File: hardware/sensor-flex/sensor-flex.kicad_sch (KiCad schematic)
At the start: 34 parts, among them IC1 VCNL4040M3OE, IC2 VCNL4040M3OE, J1 Conn_01x05, U1 PCA9546APWR

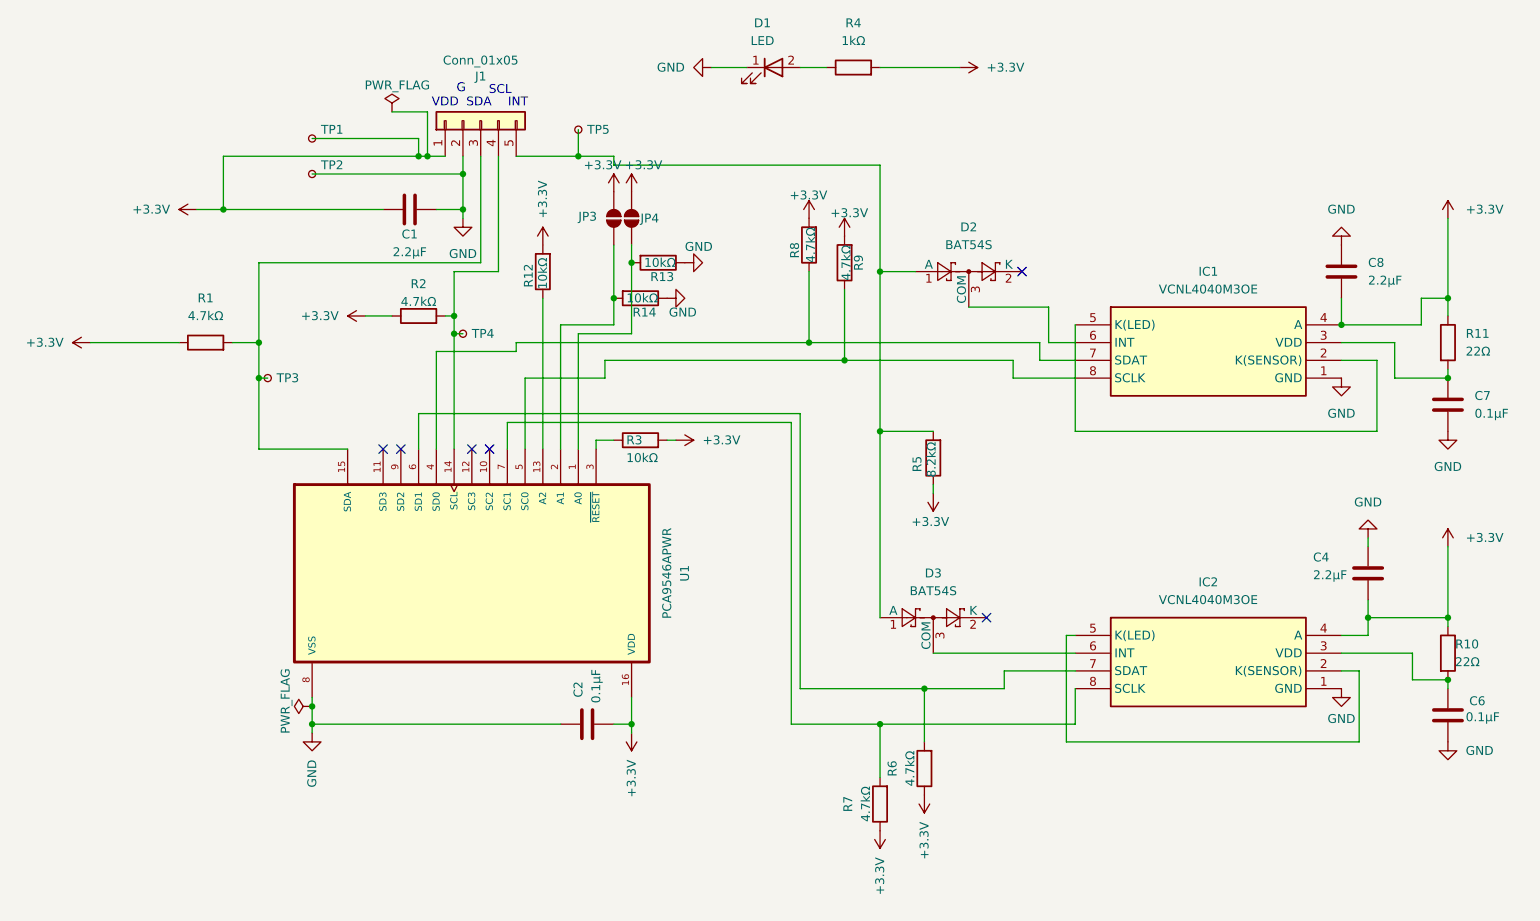
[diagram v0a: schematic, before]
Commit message: Interrupts and new flex design
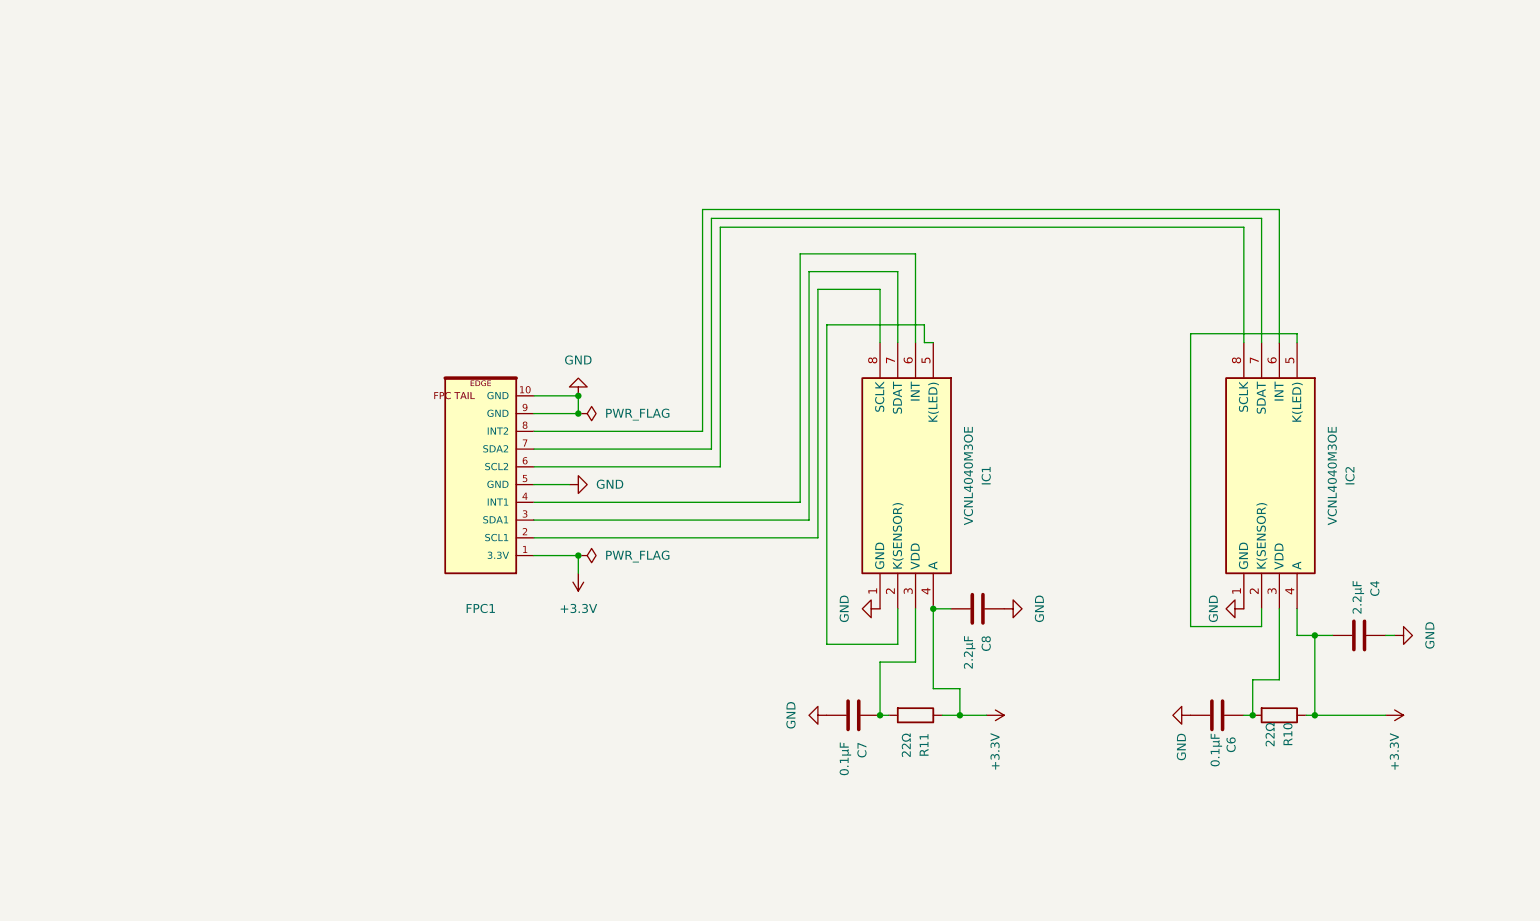
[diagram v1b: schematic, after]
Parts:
- removed C1: 2.2µF, Capacitor_SMD:C_0603_1608Metric, symbol Device:C
- removed C2: 0.1µF, Capacitor_SMD:C_0603_1608Metric, symbol Device:C
- removed D1: LED, LED_SMD:LED_0603_1608Metric, symbol Device:LED
- removed D2, D3: BAT54S, Package_TO_SOT_SMD:SOT-23, symbol Diode:BAT54S
- removed J1: Conn_01x05, Connector_JST:JST_SH_SM05B-SRSS-TB_1x05-1MP_P1.00mm_Horizontal, symbol Connector_Generic:Conn_01x05
- removed JP3, JP4: SolderJumper_2_Open, Jumper:SolderJumper-2_P1.3mm_Open_RoundedPad1.0x1.5mm, symbol Jumper:SolderJumper_2_Open
- removed R1, R2, R6, R7, R8, R9: 4.7kΩ, Resistor_SMD:R_0603_1608Metric, symbol Device:R
- removed R12, R13, R14, R3: 10kΩ, Resistor_SMD:R_0603_1608Metric, symbol Device:R
- removed R4: 1kΩ, Resistor_SMD:R_0603_1608Metric, symbol Device:R
- removed R5: 8.2kΩ, Resistor_SMD:R_0603_1608Metric, symbol Device:R
- removed TP1, TP2, TP3, TP4, TP5: TestPoint_Small, TestPoint:TestPoint_Pad_D1.5mm, symbol Connector:TestPoint_Small
- removed U1: PCA9546APWR, motion-play-footprints:SOP65P640X120-16N, symbol motion-play-symbols:PCA9546APWR
- added FPC1: FPC_Tail_10P, motion-play-footprints:FPC_Tail_10P_1.0mm_TopContact, symbol motion-play-symbols:FPC_Tail_10P
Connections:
- net +3.3V: now also FPC1.1 (3.3V)
- net GND: now also FPC1.10 (GND), FPC1.5 (GND), FPC1.9 (GND)
- net at IC1.7 (SDAT): now also FPC1.3 (SDA1)
- net at IC1.8 (SCLK): now also FPC1.2 (SCL1)
- net at IC2.7 (SDAT): now also FPC1.7 (SDA2)
- net at IC2.8 (SCLK): now also FPC1.6 (SCL2)
- net at IC2.6 (INT): now also FPC1.8 (INT2)
- net at IC1.6 (INT): now also FPC1.4 (INT1)
- no-connect marks 6 -> 0
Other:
- note removed: "G"
- note removed: "INT"
- note removed: "SCL"
- note removed: "SDA"
- note removed: "VDD"
- moved on the sheet: C4, C6, C7, C8, IC1, IC2, R10, R11

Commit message: Generate circuit-context.json for sensor-rigid and sensor-flex PCBs
Run the existing schematic context extraction and annotation tooling on
both sensor board schematics. Sensor-rigid: 27 components, 16 nets,
6 functional blocks (i2c_mux, connectors, i2c_pull_ups, interrupts,
power, test_points). Sensor-flex: 9 components, 12 nets, 4 blocks
(sensor_1, sensor_2, power, connector). All ai_ properties written to
.kicad_sch files for persistence. Initiative docs and status updates
included.

Made-with: Cursor
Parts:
- C4: ai_block (none) -> power; ai_critical_specs (none) -> 2.2µF, 0603; ai_function (none) -> IR LED supply bypass capacitor for sensor 1; ai_role (none) -> bypass
- C6: ai_block (none) -> sensor_2; ai_critical_specs (none) -> 0.1µF, 0603; ai_function (none) -> VDD bypass capacitor for sensor 2; ai_role (none) -> bypass
- C7: ai_block (none) -> sensor_1; ai_critical_specs (none) -> 0.1µF, 0603; ai_function (none) -> VDD bypass capacitor for sensor 1; ai_role (none) -> bypass
- C8: ai_block (none) -> power; ai_critical_specs (none) -> 2.2µF, 0603; ai_function (none) -> IR LED supply bypass capacitor for sensor 2; ai_role (none) -> bypass
- FPC1: ai_block (none) -> connector; ai_critical_specs (none) -> 10-pin, 1.0mm pitch, top contact; ai_function (none) -> FPC tail connector mating with ZIF on rigid base — carries 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; ai_role (none) -> connector
- IC1: ai_block (none) -> sensor_1; ai_critical_specs (none) -> VCNL4040M3OE, I2C 0x60, 400kHz; ai_function (none) -> Proximity and ambient light sensor 1 (Side A); ai_role (none) -> sensor
- IC2: ai_block (none) -> sensor_2; ai_critical_specs (none) -> VCNL4040M3OE, I2C 0x60, 400kHz; ai_function (none) -> Proximity and ambient light sensor 2 (Side B); ai_role (none) -> sensor
- R10: ai_block (none) -> sensor_2; ai_critical_specs (none) -> 22Ω, 0603; ai_function (none) -> VDD series filter resistor for sensor 2; ai_role (none) -> filter
- R11: ai_block (none) -> sensor_1; ai_critical_specs (none) -> 22Ω, 0603; ai_function (none) -> VDD series filter resistor for sensor 1; ai_role (none) -> filter

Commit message: Hardware revision: remove interrupts, update connectors, add DIP switch
Remove INT lines from all three PCBs (main, rigid, flex). Replace 5-pin
JST-SH connectors with 4-pin SM04B-SRSS-TB on main and rigid boards.
Replace solder jumpers with EP-02KS DIP switch for I2C address config
on rigid board. Update FPC connector pinout to remove INT signals and
add GND fills. Update stiffener specs (PI 0.25mm tail, SS 0.2mm IC
areas). Regenerate production files (BOM, CPL) for both sensor boards.
Update hardware CONTEXT.md with corrected addresses (0x74-0x76),
component tables, and pinouts.

Made-with: Cursor
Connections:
- net +3.3V: now also R10.2; no longer R10.1
- net GND: now also FPC1.2 (GND), FPC1.8 (GND)
- net VDD_S2: now reaches C6.1, IC2.3 (VDD)
- net VDD_S2: now also R10.1; no longer R10.2
- net LED_K2: now reaches IC2.2 (K(SENSOR)), IC2.5 (K(LED))
- net at IC2.6 (INT): no longer FPC1.8 (INT2)
- net SDA2: now reaches FPC1.7 (SDA2), IC2.7 (SDAT)
- net SCL2: now reaches FPC1.6 (SCL2), IC2.8 (SCLK)
- net SCL1: now reaches IC1.8 (SCLK)
- net SCL1: now also FPC1.3 (SCL1); no longer FPC1.2 (SCL1)
- net SDA1: now reaches IC1.7 (SDAT)
- net SDA1: now also FPC1.4 (SDA1); no longer FPC1.3 (SDA1)
- net at IC1.6 (INT): no longer FPC1.4 (INT1)
- net VDD_S1: now reaches C7.1, IC1.3 (VDD), R11.2
- net LED_K1: now reaches IC1.2 (K(SENSOR)), IC1.5 (K(LED))
- no-connect marks 0 -> 2
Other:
- moved on the sheet: IC1, IC2
